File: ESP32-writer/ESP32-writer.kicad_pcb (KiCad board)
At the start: 2 copper layers, 27.2 x 30.6 mm, 17 parts, among them J1 USB2.0_C, J2 UART-OUTPUT, J3 USB2.0_C, Q1 2N7002, Q2 2N7002, U1 CH340C

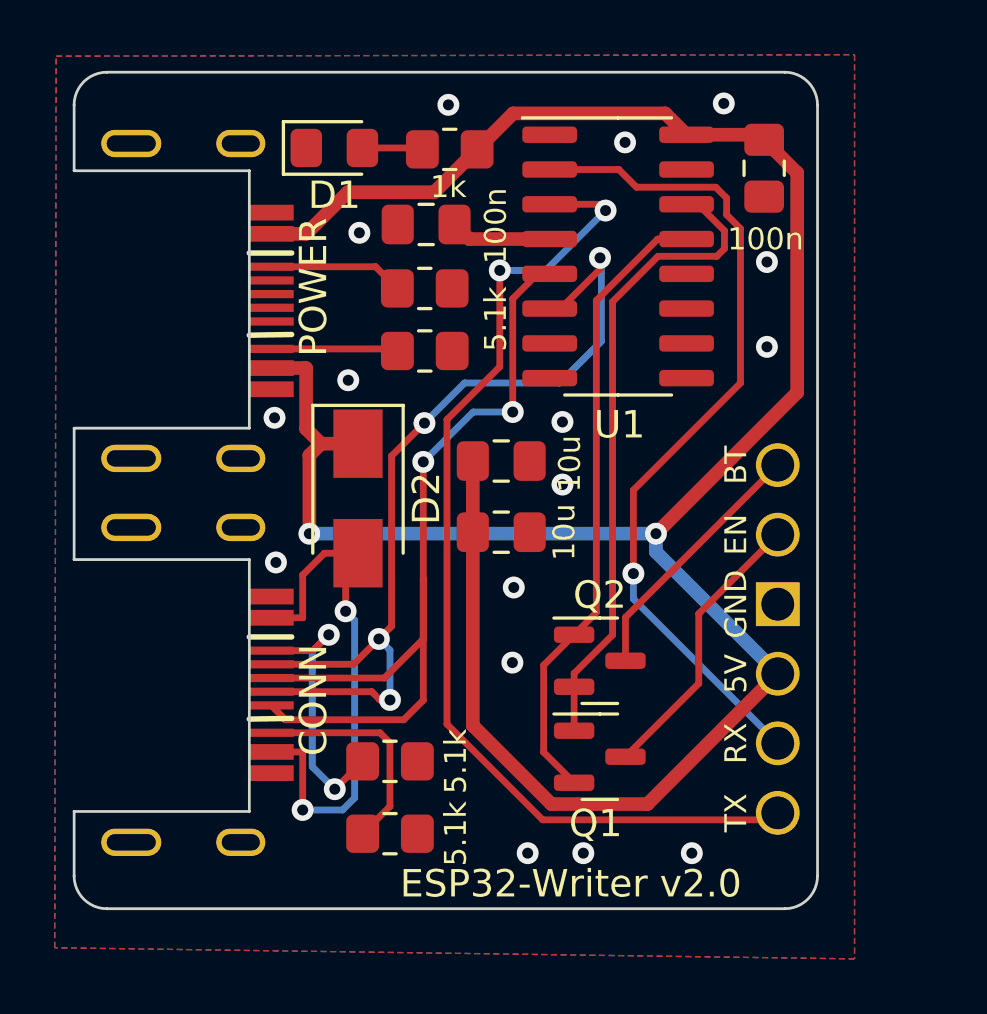
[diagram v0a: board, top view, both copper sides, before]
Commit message: up
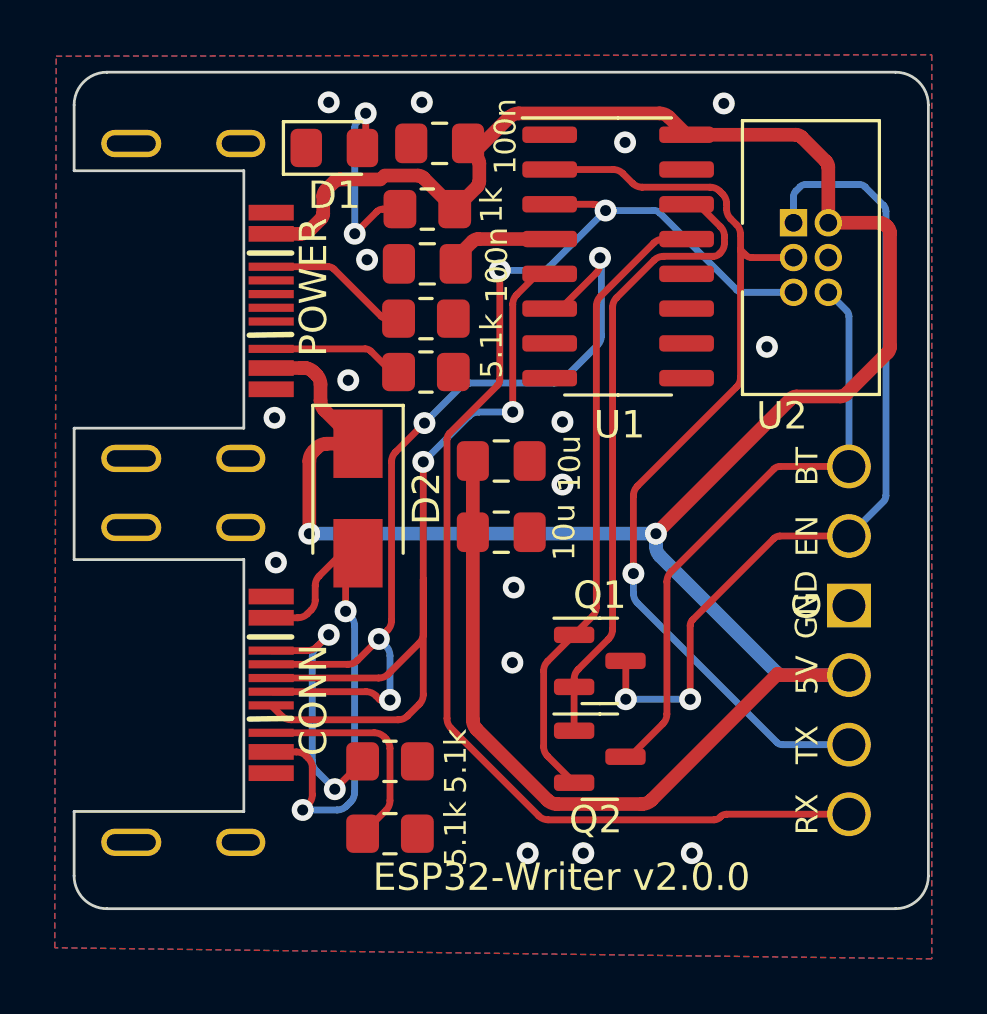
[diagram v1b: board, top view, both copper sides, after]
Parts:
- added U2: ESP-Prog-ProgramCOM-SEND, $74th:BoxPinHeader_2x03_P1.27mm_Vertical, F.Cu at (93.9, 68.6)
- moved C3 11.9 mm to (80.3, 64.4), turned to 180 degrees
- moved Q2 3.51 mm to (86.2, 86.8)
- moved Q1 3.50 mm to (86.2, 83.3)
- moved J2 2.60 mm to (94.0, 90.2)
- moved R3 2.33 mm to (79.8, 66.9)
- moved C2 1.44 mm to (79.9, 68.8)
- moved R1 1.10 mm to (80.0, 70.7)
- moved R2 0.77 mm to (80.0, 72.7)
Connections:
- Q1 pad 1: RTS -> DTR
- Q1 pad 2: DTS -> RTS
- Q2 pad 1: DTS -> RTS
- Q2 pad 2: RTS -> DTR
- U1 pad 13: DTS -> DTR
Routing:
- net DTS: track 23.1 -> 0.00 mm
- net DTR: track 0.00 -> 23.0 mm
- net RESET: track 10.4 -> 31.1 mm, vias 0 -> 2
- net +5V: track 89.9 -> 103.7 mm
- net BOOT: track 9.45 -> 22.2 mm
- net RXD: track 37.9 -> 48.4 mm
- net Net-(D1-Pad2): track 2.21 -> 7.86 mm, vias 0 -> 2
- net TXD: track 30.8 -> 35.3 mm
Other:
- board size 27.2 x 30.6 mm -> 31.2 x 30.5 mm
- board text added: "ESP32-Writer v2.0.0"
- board text added: "JLCJLCJLCJLC"
- board text removed: "ESP32-Writer v2.0"
